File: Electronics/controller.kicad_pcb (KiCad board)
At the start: 2 copper layers, 120 x 65 mm, 66 parts, among them J501 Conn_01x06_Female, J502 Conn_01x06_Female, Q201 IRLZ44N, Q202 IRLIZ44N, Q203 IRLZ44N, Q204 IRLIZ44N, Q205 IRLZ44N, Q206 IRLIZ44N, U201 74LS08, U202 IR2101, U203 IR2101, U204 IR2101, U401 R-78B15-2.0, U402 R-78E3.3-1.0

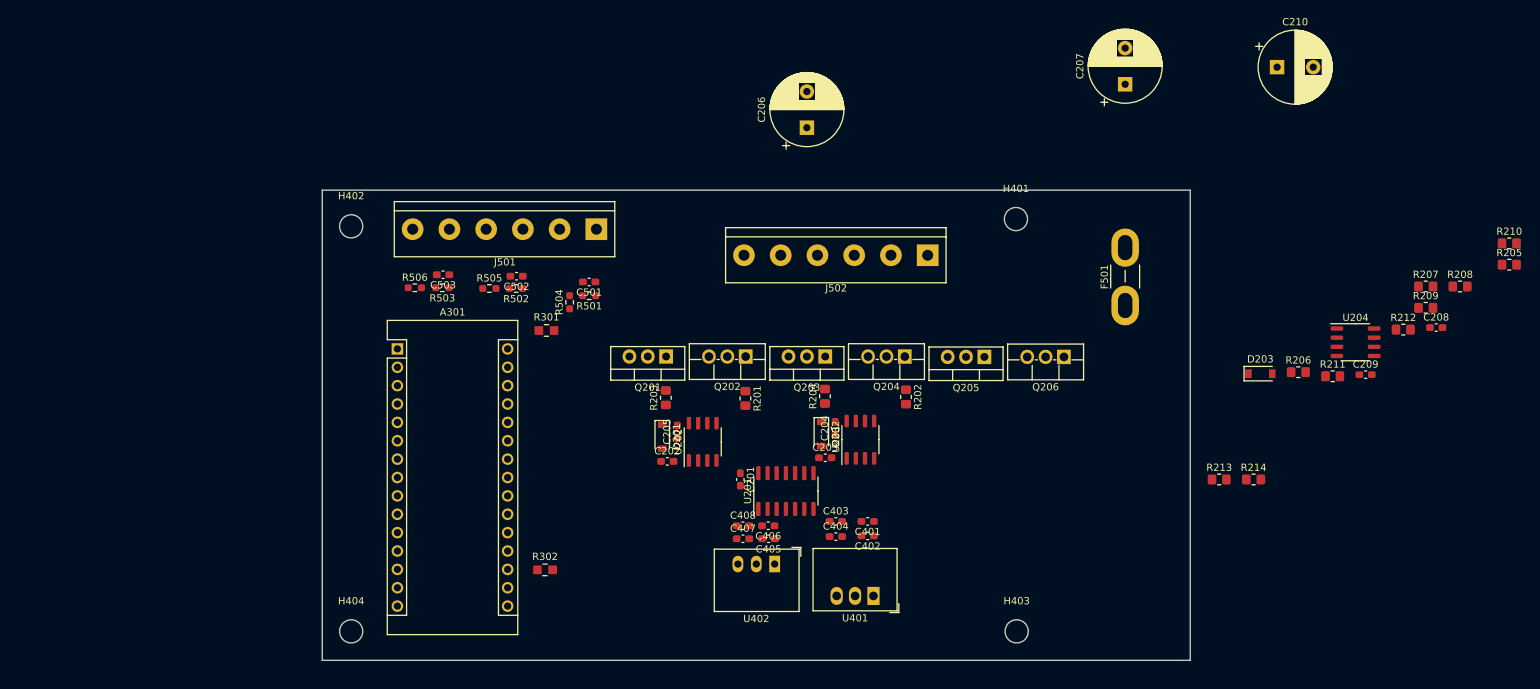
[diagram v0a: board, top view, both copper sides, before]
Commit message: Layout update
Signed-off-by: Aki Kuusela <git@findersee.fi>
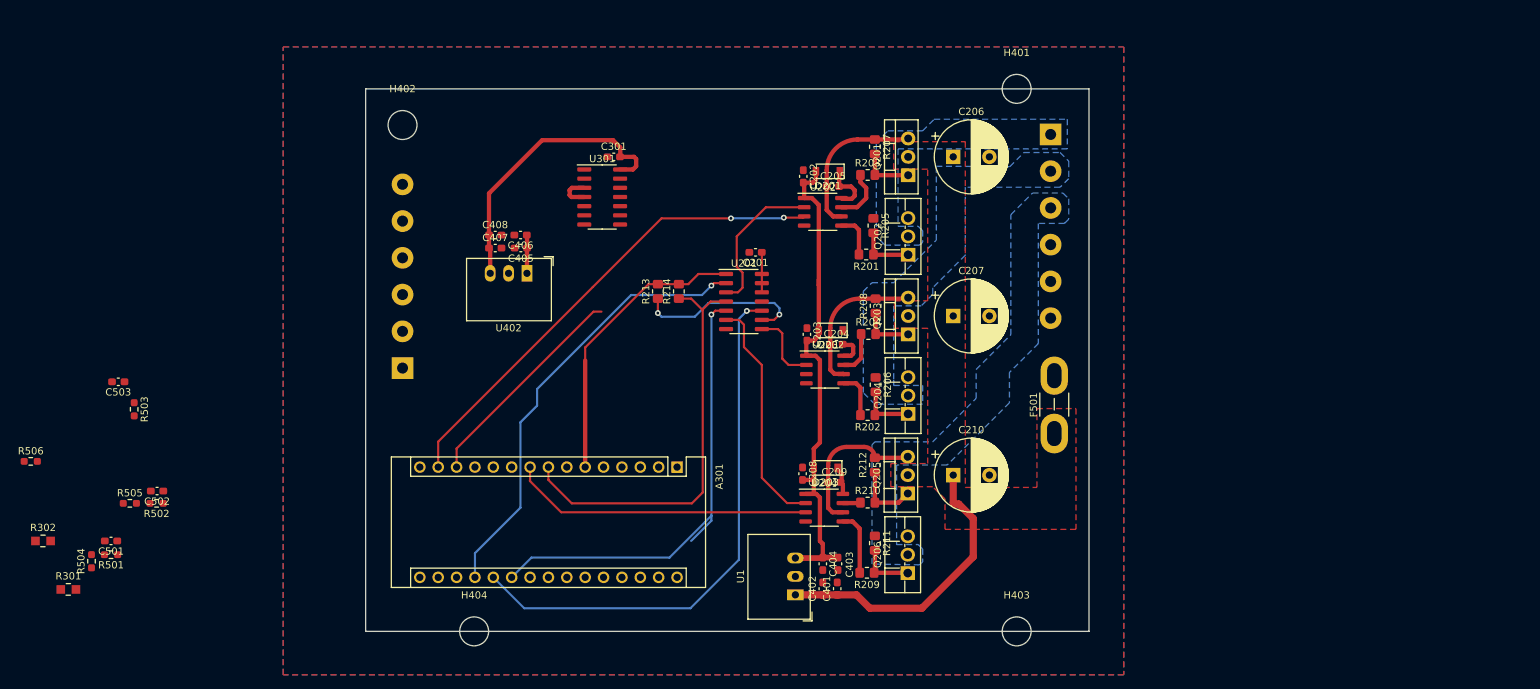
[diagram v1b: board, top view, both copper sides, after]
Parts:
- removed U401: R-78B15-2.0, Converter_DCDC:Converter_DCDC_RECOM_R-78B-2.0_THT
- added C301: 100n, Capacitor_SMD:C_0603_1608Metric_Pad1.08x0.95mm_HandSolder, F.Cu at (111.3, 62.4)
- added U1: R-78C15-1.0, Converter_DCDC:Converter_DCDC_RECOM_R-78E-0.5_THT, F.Cu at (136.4, 122.9)
- added U301: 74HC86, Package_SO:SO-14_3.9x8.65mm_P1.27mm, F.Cu at (109.7, 68.0)
- H401, H402, H403, H404: footprint MountingHole:MountingHole_3.2mm_M3 -> MountingHole:MountingHole_4mm
- J501: moved to B.Cu
- J502: value Conn_01x06_Female -> Motor Con; moved to B.Cu
- moved R210 95.7 mm to (146.4, 110.2)
- moved C208 89.9 mm to (137.4, 106.2), turned to -90 degrees
- moved R205 88.1 mm to (147.2, 71.9), turned to -90 degrees
- moved R209 85.5 mm to (146.3, 119.9), turned to 180 degrees
- moved R214 83.6 mm to (120.3, 81.0), turned to 90 degrees
- moved R213 81.8 mm to (117.4, 81.0), turned to 90 degrees
- moved R208 80.8 mm to (147.5, 83.0), turned to 90 degrees
- moved R207 78.6 mm to (147.4, 61.0), turned to -90 degrees
- moved U204 76.9 mm to (140.4, 110.9)
- moved R212 75.4 mm to (147.4, 105.0), turned to 90 degrees
- moved R501 75.2 mm to (41.8, 117.4)
- moved C501 75.2 mm to (41.8, 115.5)
- moved R301 75.2 mm to (35.9, 122.2)
- moved R504 75.2 mm to (39.1, 118.3)
- moved C209 74.9 mm to (141.8, 107.4)
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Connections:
- J502 pad 1: Net-(F501-Pad2) -> /Connectors/MOTOR POS
- J502 pad 2: GND -> /Connectors/MOTOR NEG
- J502 pad 3: unconnected-(J502-Pad3) -> /Connectors/MOTOR C
- J502 pad 4: /Connectors/MOTOR C -> unconnected-(J502-Pad4)
- J502 pad 5: /Connectors/MOTOR NEG -> GND
- J502 pad 6: /Connectors/MOTOR POS -> Net-(F501-Pad2)
- U201 pad 10: +3V3 -> /Connectors/Limit 2
- U201 pad 11: Net-(U201-Pad11) -> unconnected-(U201-Pad11)
- U201 pad 12: /Hbridge/HIN C -> +3V3
- U201 pad 13: /Hbridge/C LIMIT -> +3V3
- U201 pad 4: /Hbridge/HIN B -> /Hbridge/HIN C
- U201 pad 5: /Connectors/Limit 2 -> /Hbridge/C LIMIT
- U201 pad 8: unconnected-(U201-Pad8) -> Net-(U201-Pad8)
- U201 pad 9: +3V3 -> /Hbridge/HIN B
- U203 pad 2: Net-(U201-Pad6) -> Net-(U201-Pad8)
- U204 pad 2: Net-(U201-Pad11) -> Net-(U201-Pad6)
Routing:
- net /Connectors/Limit 2: track 0.00 -> 75.4 mm, vias 0 -> 1
- net VCC: track 0.00 -> 75.1 mm
- net /Hbridge/LIN A: track 0.00 -> 67.0 mm, vias 0 -> 2
- net /Hbridge/C LIMIT: track 0.00 -> 65.8 mm, vias 0 -> 1
- net /Connectors/Limit 1: track 0.00 -> 61.8 mm, vias 0 -> 1
- net /Hbridge/HIN C: track 0.00 -> 58.0 mm
- net /Hbridge/HIN A: track 0.00 -> 55.0 mm
- net /Hbridge/HIN B: track 0.00 -> 54.1 mm, vias 0 -> 2
- net +3V3: track 0.00 -> 45.3 mm
- net /Hbridge/LIN C: track 0.00 -> 41.8 mm
- net Vdrive: track 0.00 -> 41.1 mm
- net Net-(U201-Pad6): track 0.00 -> 32.4 mm
- net /Connectors/MOTOR POS: track 0.00 -> 21.5 mm
- net /Connectors/MOTOR C: track 0.00 -> 21.4 mm
- net Net-(U201-Pad3): track 0.00 -> 21.0 mm
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- added copper zone on B.Cu, net /Connectors/MOTOR C
- added copper zone on B.Cu, net /Connectors/MOTOR NEG
- added copper zone on B.Cu, net /Connectors/MOTOR POS
- added copper zone on B.Cu, net GND
- added copper zone on F.Cu, net GND
- added copper zone on F.Cu, net Vdrive
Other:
- board size 120 x 65 mm -> 100 x 75 mm
